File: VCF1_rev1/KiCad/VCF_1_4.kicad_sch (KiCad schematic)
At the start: 32 parts, among them U3 CEM3350, U4 Opamp_Quad

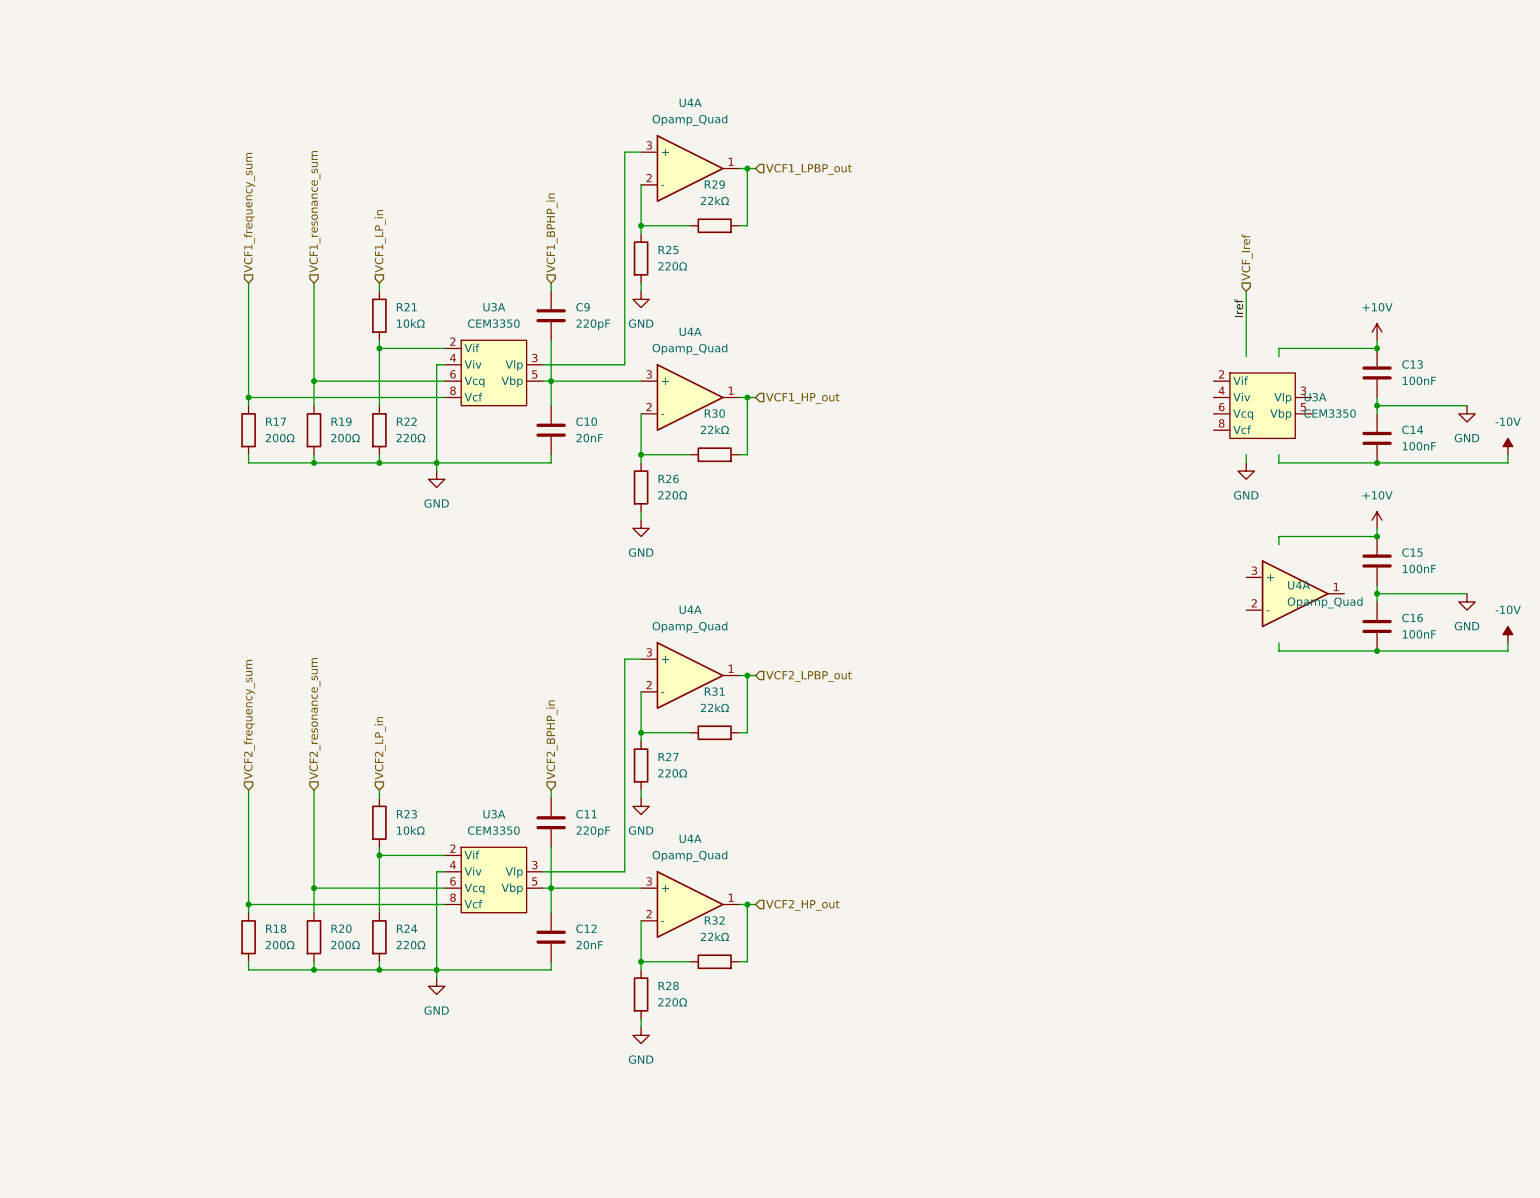
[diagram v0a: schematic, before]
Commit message: A lot of work especially on VCF2. Doc updated. Schematics a bit in a flux due to major restructuring.
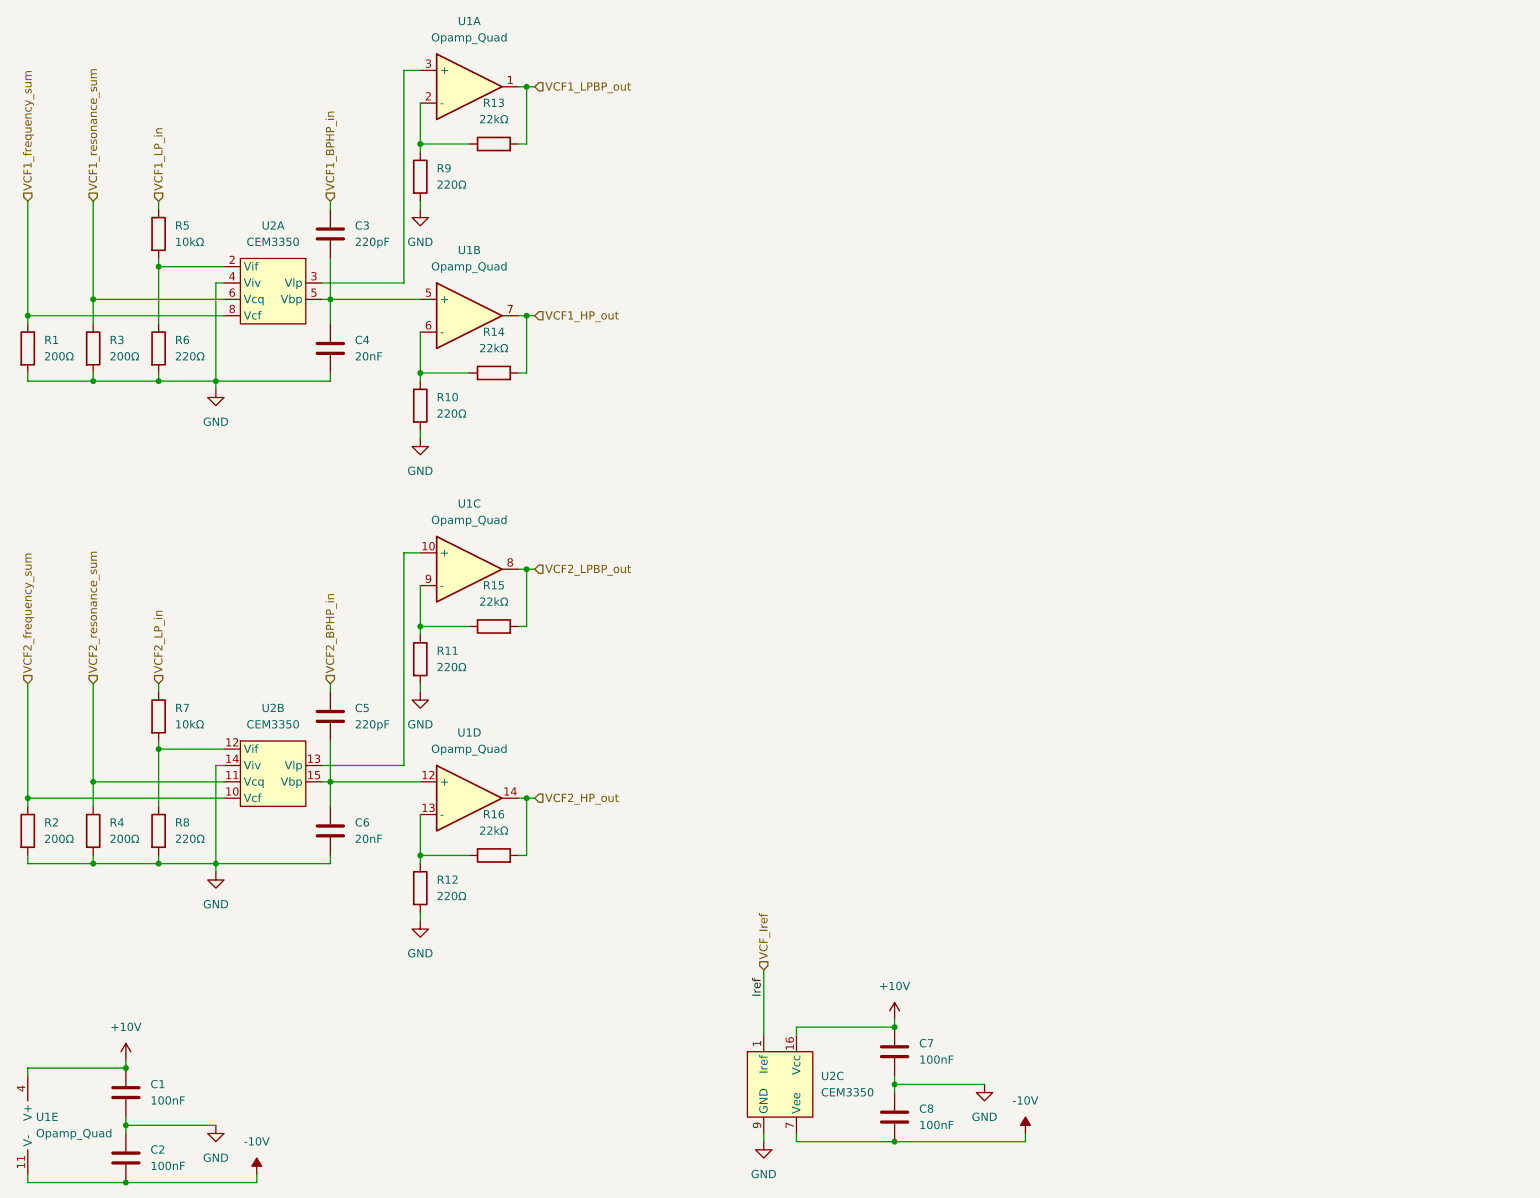
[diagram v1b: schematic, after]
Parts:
- removed C10, C12: 20nF, symbol Device:C
- removed C11, C9: 220pF, symbol Device:C
- removed C13, C14, C15, C16: 100nF, symbol Device:C
- removed R17, R18, R19, R20: 200Ω, symbol Device:R
- removed R21, R23: 10kΩ, symbol Device:R
- removed R22, R24, R25, R26, R27, R28: 220Ω, symbol Device:R
- removed R29, R30, R31, R32: 22kΩ, symbol Device:R
- removed U3 (x3): CEM3350, symbol Modular_Mayhem:CEM3350
- removed U4 (x5): Opamp_Quad, symbol Device:Opamp_Quad
- added C1, C2, C7, C8: 100nF, symbol Device:C
- added C3, C5: 220pF, symbol Device:C
- added C4, C6: 20nF, symbol Device:C
- added R1, R2, R3, R4: 200Ω, symbol Device:R
- added R10, R11, R12, R6, R8, R9: 220Ω, symbol Device:R
- added R13, R14, R15, R16: 22kΩ, symbol Device:R
- added R5, R7: 10kΩ, symbol Device:R
- added U1: Opamp_Quad, symbol Device:Opamp_Quad
- added U2: CEM3350, symbol Modular_Mayhem:CEM3350
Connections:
- net +10V: now also C1.1, C7.1, U1.4 (V+), U2.16 (Vcc)
- net -10V: now also C2.2, C8.2, U1.11 (V-), U2.7 (Vee)
- net GND: now also C1.2, C2.1, C4.2, C6.2, C7.2, C8.1, R1.2, R10.2, R11.2, R12.2, R2.2, R3.2, R4.2, R6.2, R8.2, R9.2, U2.14 (Viv), U2.4 (Viv), U2.9 (GND)
- net VCF1_BPHP_in: now also C3.1
- net VCF1_HP_out: now also R14.2, U1.7
- net VCF1_LPBP_out: now also R13.2, U1.1
- net VCF1_LP_in: now also R5.1
- net VCF1_frequency_sum: now also R1.1, U2.8 (Vcf)
- net VCF1_resonance_sum: now also R3.1, U2.6 (Vcq)
- net VCF2_BPHP_in: now also C5.1
- net VCF2_HP_out: now also R16.2, U1.14
- net VCF2_LPBP_out: now also R15.2, U1.8
- net VCF2_LP_in: now also R7.1
- net VCF2_frequency_sum: now also R2.1, U2.10 (Vcf)
- net VCF2_resonance_sum: now also R4.1, U2.11 (Vcq)
- net VCF_Iref: now also U2.1 (Iref)
- new net: C3.2, C4.1, U1.5 (+), U2.5 (Vbp)
- new net: C5.2, C6.1, U1.12 (+), U2.15 (Vbp)
- new net: R10.1, R14.1, U1.6 (-)
- new net: R7.2, R8.1, U2.12 (Vif)
- new net: U1.10 (+), U2.13 (Vlp)
- new net: R13.1, R9.1, U1.2 (-)
- new net: U1.3 (+), U2.3 (Vlp)
- new net: R5.2, R6.1, U2.2 (Vif)
- new net: R12.1, R16.1, U1.13 (-)
- new net: R11.1, R15.1, U1.9 (-)
